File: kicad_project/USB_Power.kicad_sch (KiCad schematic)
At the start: 36 parts, among them J3 USB_C_Receptacle_USB2.0, J4 Conn_01x01, Q1 DMP2104LP, Q2 DMP2104LP, Q3 HSCC8233, Q4 TPM3134NX3, Q5 DMP2104LP, U3 SRV05-4, U4 TP4056, U5 DW01x, U6 NCP167BMX330TBG, U7 NCP167BMX330TBG

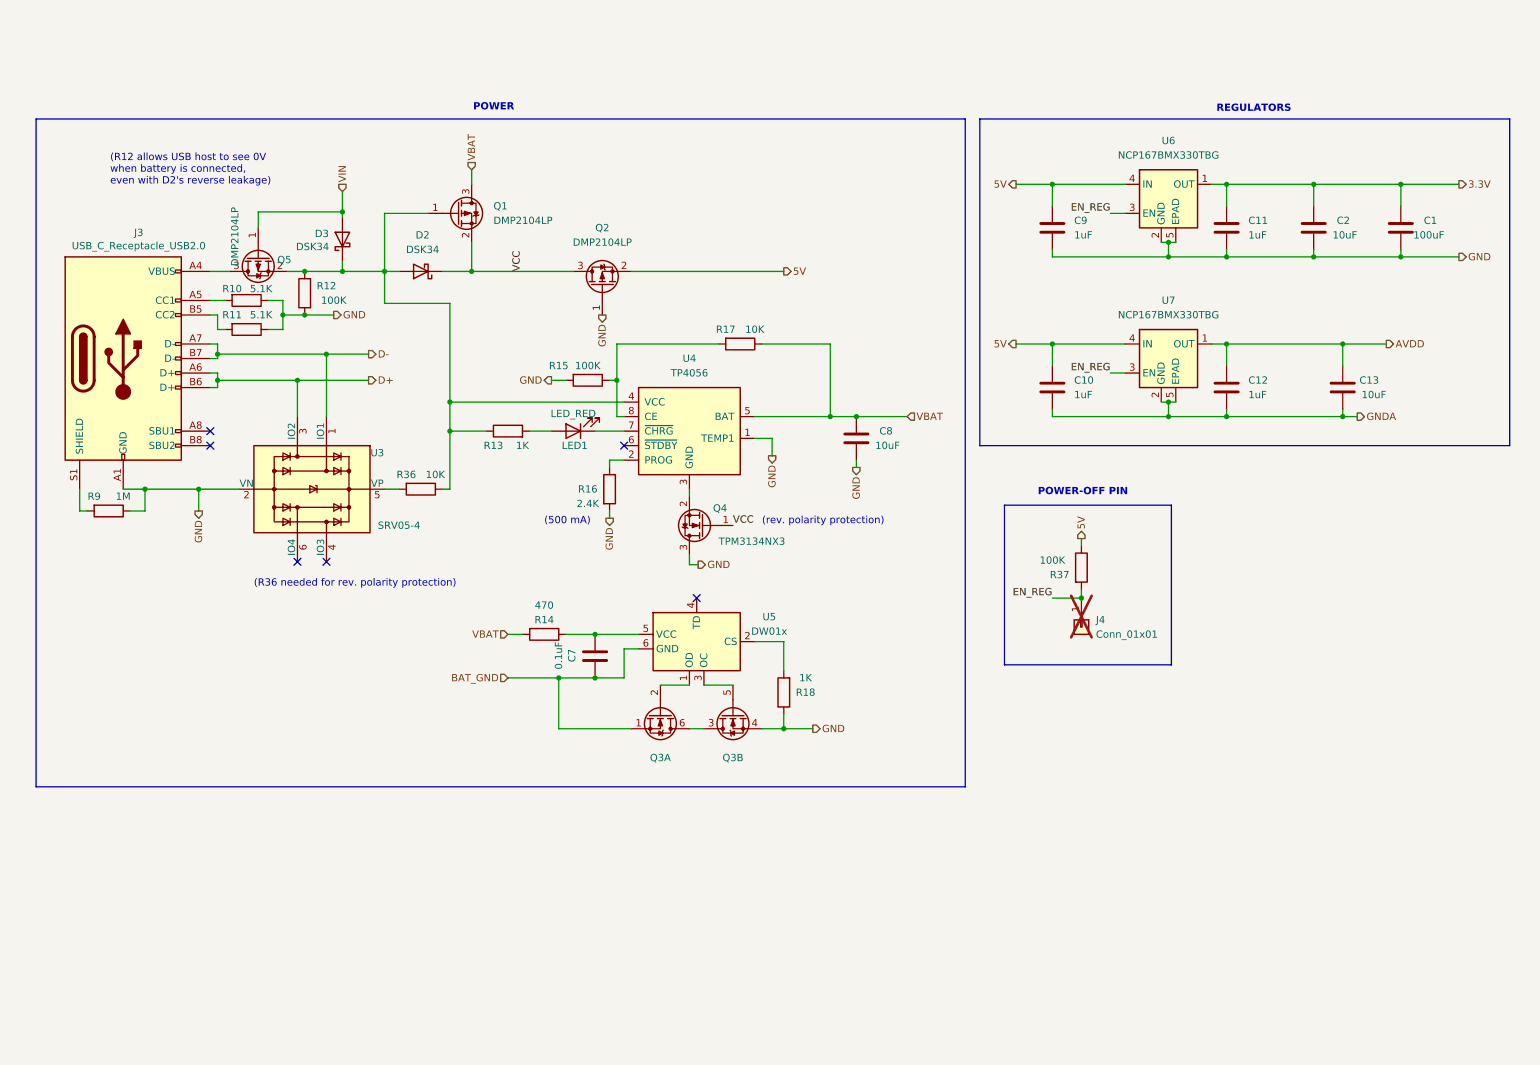
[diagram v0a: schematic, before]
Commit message: Initial commit
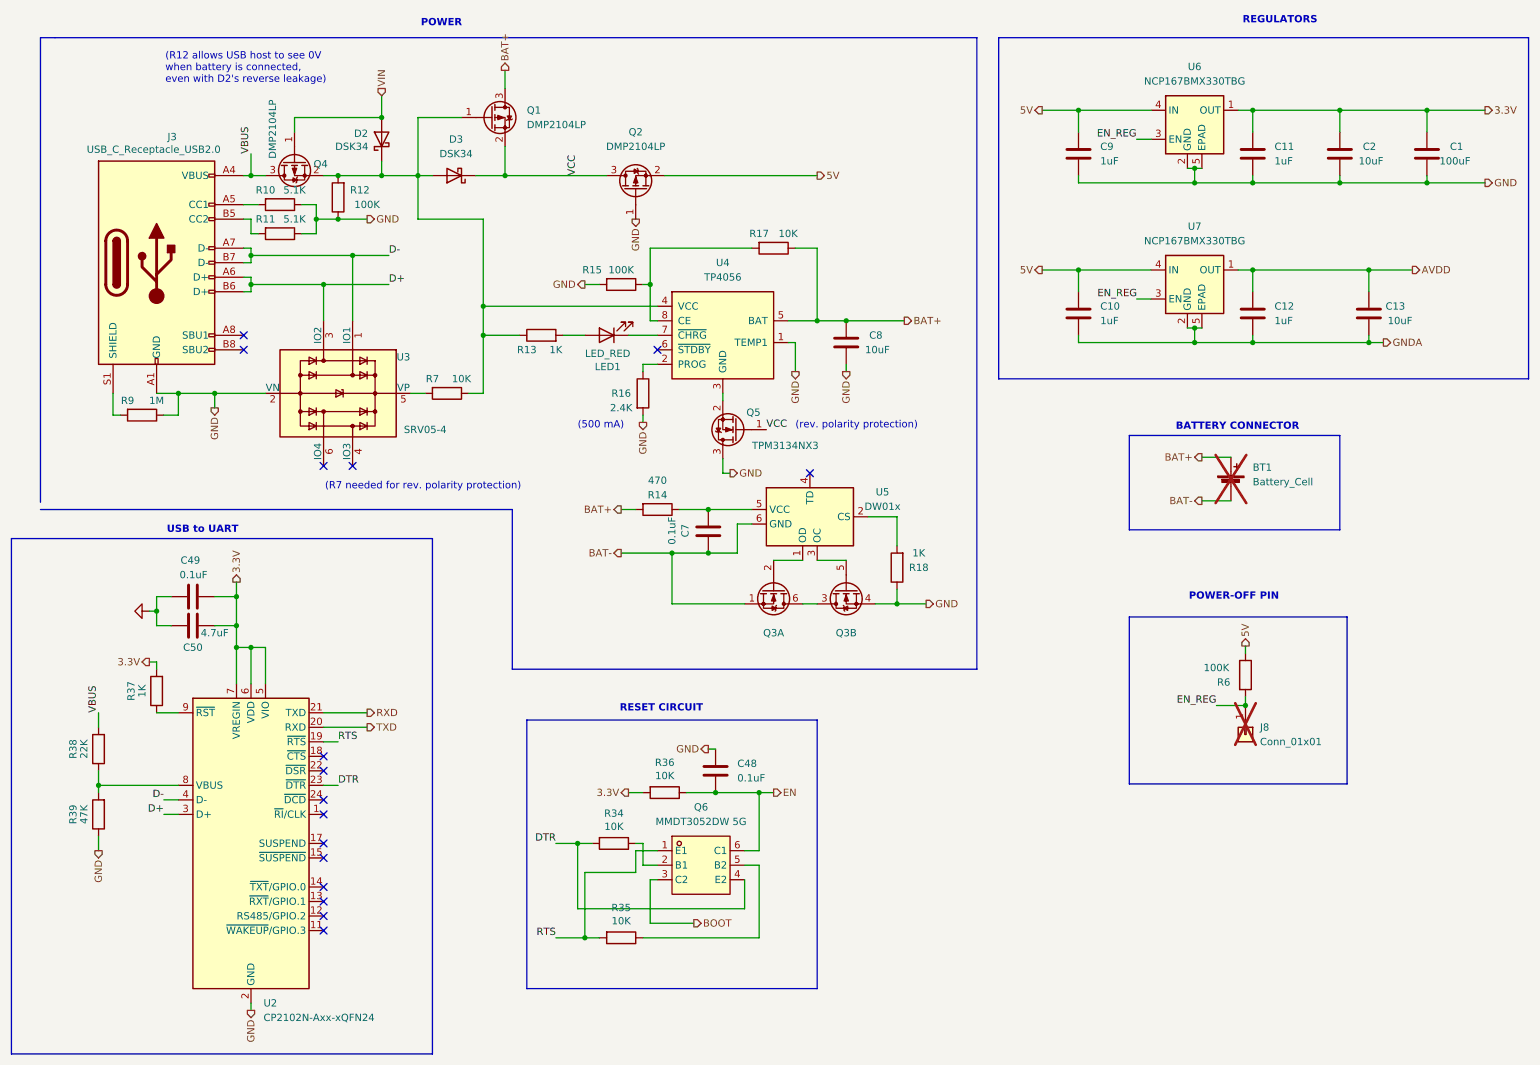
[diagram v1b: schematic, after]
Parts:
- removed J4: Conn_01x01, Connector_PinHeader_2.54mm:PinHeader_1x01_P2.54mm_Vertical, symbol Connector_Generic:Conn_01x01
- removed Q4: TPM3134NX3, Package_TO_SOT_SMD:SOT-723, symbol Device:Q_NMOS_GSD
- removed Q5: DMP2104LP, Custom:Diodes_DFN1411-3, symbol Device:Q_PMOS_GSD
- added BT1: Battery_Cell, Connector_JST:JST_PH_S2B-PH-SM4-TB_1x02-1MP_P2.00mm_Horizontal, symbol Device:Battery_Cell
- added C48, C49: 0.1uF, Capacitor_SMD:C_0402_1005Metric, symbol Device:C
- added C50: 4.7uF, Capacitor_SMD:C_0402_1005Metric, symbol Device:C
- added J8: Conn_01x01, Connector_PinHeader_2.54mm:PinHeader_1x01_P2.54mm_Vertical, symbol Connector_Generic:Conn_01x01
- added Q4: DMP2104LP, Custom:Diodes_DFN1411-3, symbol Device:Q_PMOS_GSD
- added Q5: TPM3134NX3, Package_TO_SOT_SMD:SOT-723, symbol Device:Q_NMOS_GSD
- added Q6: MMDT3052DW 5G, Package_TO_SOT_SMD:SOT-363_SC-70-6, symbol Custom:MMDT3052DW5G
- added R34, R35, R7: 10K, Resistor_SMD:R_0402_1005Metric, symbol Device:R
- added R38: 22K, Resistor_SMD:R_0402_1005Metric, symbol Device:R
- added R39: 47K, Resistor_SMD:R_0402_1005Metric, symbol Device:R
- added R6: 100K, Resistor_SMD:R_0402_1005Metric, symbol Device:R
- added U2: CP2102N-Axx-xQFN24, Package_DFN_QFN:QFN-24-1EP_4x4mm_P0.5mm_EP2.6x2.6mm, symbol Interface_USB:CP2102N-Axx-xQFN24
- Q1, Q2: footprint Custom:Diodes_DFN1411-3 -> CustomLibrary:Diodes_DFN1411-3
- R37: value 100K -> 1K; LCSC C25741 -> C11702
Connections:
- net 3.3V: now also R36.2, R37.2, C49.2, C50.1, U2.5 (VIO), U2.6 (VDD), U2.7 (VREGIN)
- net 5V: now also R6.1; no longer R37.1
- net D+: now also U2.3 (D+)
- net D-: now also U2.4 (D-)
- net EN_REG: now also J8.1 (Pin_1), R6.2; no longer R37.2
- net GND: now also C48.1, C49.1, C50.2, Q5.3 (D), R39.1, U2.2 (GND), U2.25 (GND)
- net VCC: now also D3.1 (K), Q5.1 (G); no longer D2.1 (K)
- net VIN: now also D2.2 (A), Q4.1 (G); no longer D3.2 (A)
- net at Q1.1 (G), R12.2, R13.1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: now also D2.1 (K), D3.2 (A), Q4.2 (S), R7.1; no longer D2.2 (A), D3.1 (K), R36.1
- net at U3.5 (VP): now also R7.2; no longer R36.2
- net at U4.3 (GND): now also Q5.2 (S)
- net VBUS: now reaches J3.A4 (VBUS), J3.A9 (VBUS), J3.B4 (VBUS), J3.B9 (VBUS)
- net VBUS: now also Q4.3 (D), R38.2
- net BAT_GND renamed BAT-
- net BAT-: now also BT1.2 (-)
- net VBAT renamed BAT+
- net BAT+: now also BT1.1 (+)
- new net: R37.1, U2.9 (~{RST})
- new net: R38.1, R39.2, U2.8 (VBUS)
- new net: Q6.5 (B2), R35.1
- new net: Q6.2 (B1), R34.1
- new net BOOT: Q6.3 (C2)
- new net DTR: Q6.4 (E2), R34.2, U2.23 (~{DTR})
- new net EN: C48.2, Q6.6 (C1), R36.1
- new net RTS: Q6.1 (E1), R35.2, U2.19 (~{RTS})
- new net RXD: U2.21 (TXD)
- new net TXD: U2.20 (RXD)
- no-connect marks 6 -> 16
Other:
- note added: "(R7 needed for rev. polarity protection)"
- note added: "BATTERY CONNECTOR"
- note added: "RESET CIRCUIT"
- note added: "USB to UART"
- note removed: "(R36 needed for rev. polarity protection)"
- title: Sonatino -> Sonatino - Bluetooth Audio Edition
- moved on the sheet: C1, C10, C11, C12, C13, C2, C7, C8, C9, J3, LED1, Q1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
